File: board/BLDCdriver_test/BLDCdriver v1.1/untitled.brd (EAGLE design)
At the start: 46 x 65 mm, 26 parts, among them M1 JST-XH-03-PIN-LONG-PAD, X1 JST-XH-02-PIN-LONG-PAD, X2 JST-XH-06-PIN-ROUND-PAD, X4 JST-XH-04-PIN-ROUND-PAD

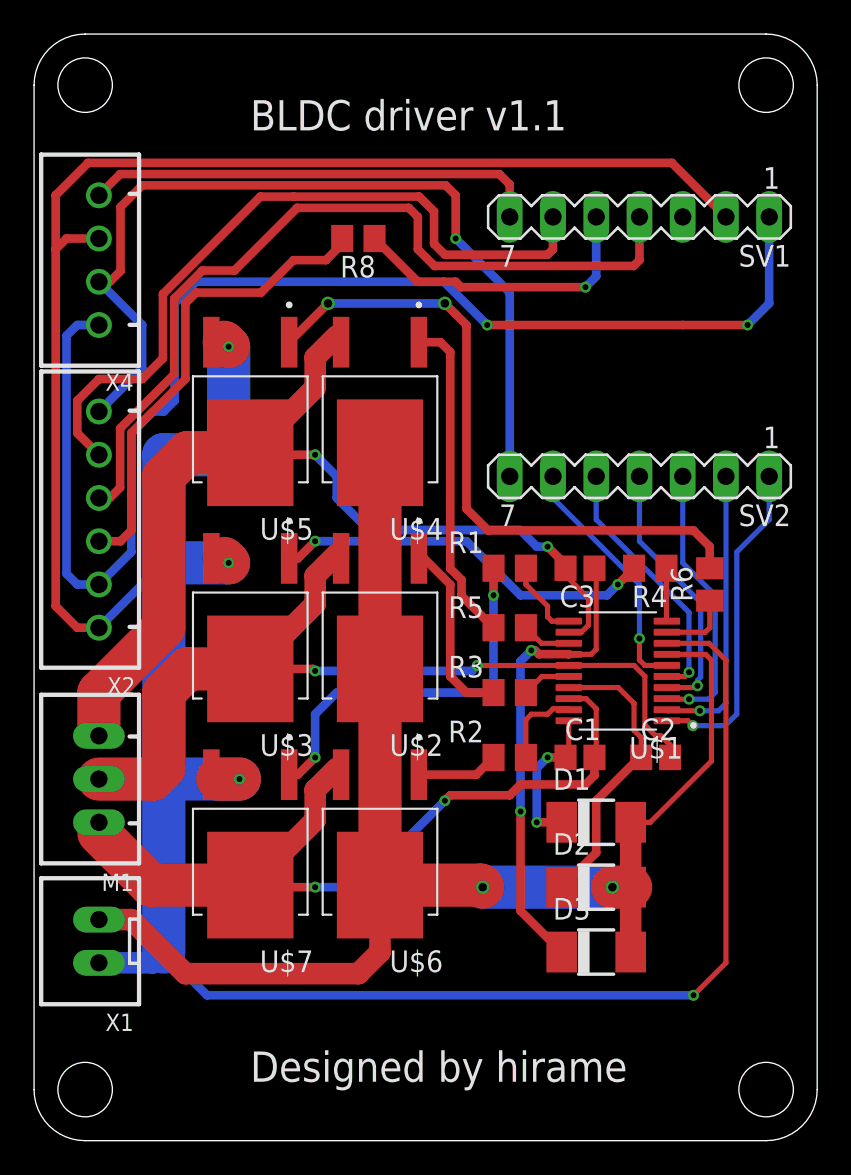
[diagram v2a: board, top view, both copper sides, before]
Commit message: Revert "Merge remote-tracking branch 'origin/Develop' into feature_#37"
This reverts commit cb103155361e8766478c6830db153463370c0739, reversing
changes made to 84e093fe944e1f8653a6822ff34e6f8740617cb5.
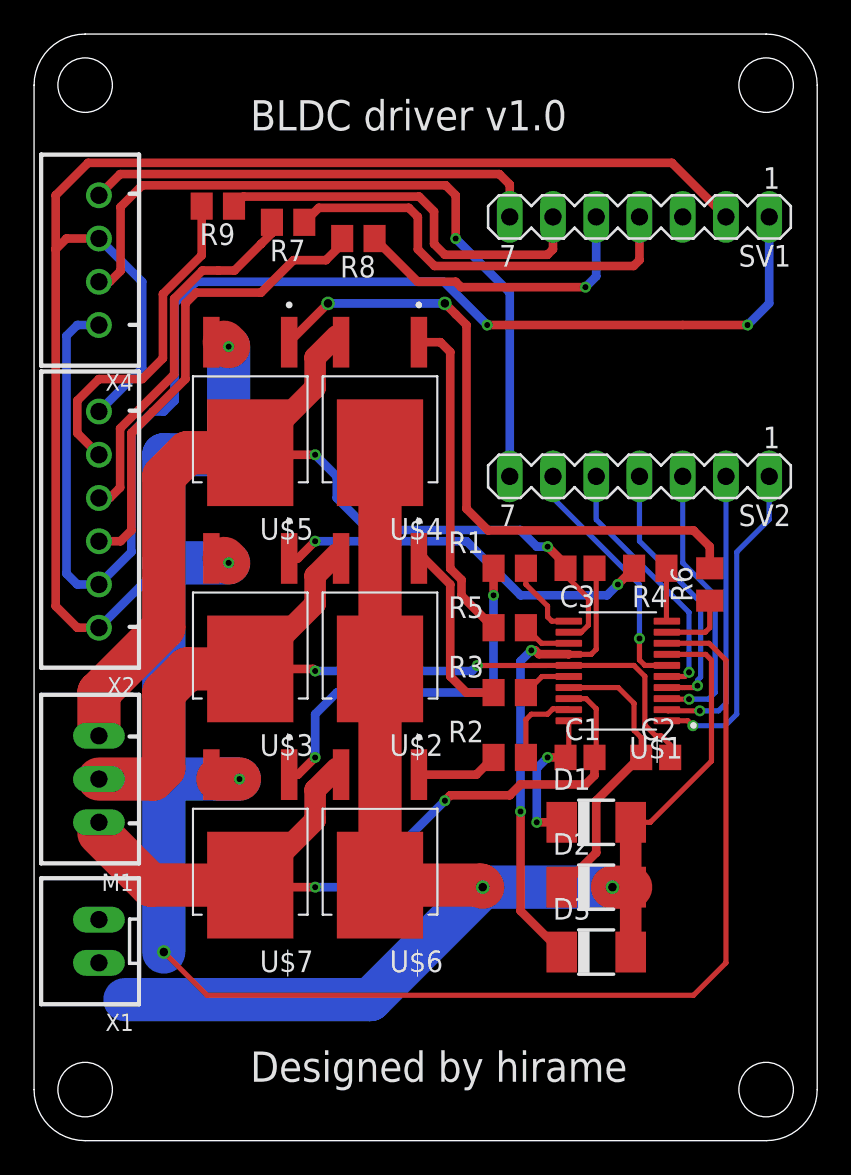
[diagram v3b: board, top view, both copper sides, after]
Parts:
- added R7, R9: 300Ω, adafruit:M2012
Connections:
- new net N$11: R7.1, SV1.4
- new net N$20: R9.1, SV1.6
- net GND: now also X2.6
- net MOSI: now also R7.2; no longer SV1.4
- net SCK: now also R9.2; no longer SV1.6
- net TX: no longer X2.6
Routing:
- net MOSI: track 48.7 -> 21.9 mm
- net N$11: track 0.00 -> 25.3 mm
- net SCK: track 43.4 -> 19.6 mm
- net N$20: track 0.00 -> 23.5 mm
- net TX: track 53.3 -> 43.6 mm
- net GND: track 188.7 -> 196.9 mm
- net VCC: track 85.0 -> 86.5 mm
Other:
- board text added: "BLDC driver v1.0"
- board text removed: "BLDC driver v1.1"
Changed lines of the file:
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@@
 <?xml version="1.0" encoding="utf-8"?>
 <!DOCTYPE eagle SYSTEM "eagle.dtd">
-<eagle version="9.6.2">
+<eagle version="9.6.1">
 <drawing>
 <settings>
@@
 <wire x1="43" y1="-6" x2="46" y2="-3" width="0.001" layer="20" curve="90"/>
 <text x="12.7" y="-2.54" size="1.778" layer="25" font="vector">Designed by hirame</text>
-<text x="12.7" y="53.34" size="1.778" layer="25" font="vector">BLDC driver v1.1</text>
+<text x="12.7" y="53.34" size="1.778" layer="25" font="vector">BLDC driver v1.0</text>
 </plain>
 <attributes>
@@
 <attribute name="VALUE" x="-0.0825" y="39.7175" size="1.016" layer="27" ratio="10" rot="R90"/>
 </element>
+<element name="R7" library="adafruit" package="M2012" value="300Ω" x="14.9225" y="47.9425" smashed="yes" rot="R180">
+<attribute name="NAME" x="15.9385" y="46.9265" size="1.27" layer="25" rot="R180"/>
+<attribute name="VALUE" x="15.9385" y="50.2285" size="1.27" layer="27" rot="R180"/>
+</element>
 <element name="R8" library="adafruit" package="M2012" value="300Ω" x="19.05" y="46.99" smashed="yes" rot="R180">
 <attribute name="NAME" x="20.066" y="45.974" size="1.27" layer="25" rot="R180"/>
 <attribute name="VALUE" x="20.066" y="49.276" size="1.27" layer="27" rot="R180"/>
+</element>
+<element name="R9" library="adafruit" package="M2012" value="300Ω" x="10.795" y="48.895" smashed="yes" rot="R180">
+<attribute name="NAME" x="11.811" y="47.879" size="1.27" layer="25" rot="R180"/>
+<attribute name="VALUE" x="11.811" y="51.181" size="1.27" layer="27" rot="R180"/>
 </element>
 </elements>
@@
 <contactref element="U$5" pad="3"/>
 <contactref element="U$1" pad="8"/>
-<wire x1="7.62" y1="15.24" x2="7.62" y2="5.08" width="2.54" layer="16"/>
+<via x="7.62" y="5.08" extent="1-16" drill="0.5"/>
+<wire x1="7.62" y1="5.08" x2="7.62" y2="15.24" width="2.54" layer="16"/>
 <wire x1="7.62" y1="15.24" x2="7.62" y2="27.94" width="2.54" layer="16"/>
 <contactref element="SV1" pad="2"/>
@@
 <wire x1="39.65" y1="23.215" x2="40.64" y2="22.225" width="0.3048" layer="1"/>
 <wire x1="40.64" y1="22.225" x2="40.64" y2="4.445" width="0.3048" layer="1"/>
+<wire x1="38.735" y1="2.54" x2="10.16" y2="2.54" width="0.3048" layer="1"/>
+<wire x1="10.16" y1="2.54" x2="7.62" y2="5.08" width="0.3048" layer="1"/>
 <wire x1="11.17" y1="40.9" x2="10.414" y2="40.9" width="0.3048" layer="1"/>
 <via x="11.43" y="40.64" extent="1-16" drill="0.35"/>
@@
 <wire x1="7.62" y1="34.29" x2="7.62" y2="27.94" width="2.54" layer="16"/>
 <wire x1="10.414" y1="15.5" x2="10.535" y2="15.5" width="0.508" layer="1"/>
+<contactref element="X2" pad="6"/>
+<wire x1="3.81" y1="46.99" x2="6.35" y2="44.45" width="0.508" layer="16"/>
+<wire x1="6.35" y1="39.37" x2="3.81" y2="36.83" width="0.508" layer="16"/>
+<wire x1="6.35" y1="44.45" x2="6.35" y2="39.37" width="0.508" layer="16"/>
 <contactref element="X1" pad="1"/>
-<wire x1="3.81" y1="4.445" x2="6.985" y2="4.445" width="1.27" layer="16"/>
-<wire x1="6.985" y1="4.445" x2="7.62" y2="5.08" width="1.27" layer="16"/>
-<wire x1="7.62" y1="5.08" x2="10.16" y2="2.54" width="0.508" layer="16"/>
-<wire x1="10.16" y1="2.54" x2="38.735" y2="2.54" width="0.508" layer="16"/>
-<via x="38.735" y="2.54" extent="1-16" drill="0.35"/>
+<wire x1="3.81" y1="4.445" x2="7.62" y2="5.08" width="0" layer="19" extent="1-1"/>
 </signal>
 <signal name="N$12">
@@
 <wire x1="39.7891" y1="22.225" x2="39.7891" y2="16.2941" width="0.3048" layer="1"/>
 <wire x1="39.7891" y1="16.2941" x2="36.195" y2="12.7" width="0.3048" layer="1"/>
+<wire x1="19.7485" y1="2.286" x2="26.3525" y2="8.89" width="2.54" layer="16"/>
+<wire x1="5.334" y1="2.286" x2="19.7485" y2="2.286" width="2.54" layer="16"/>
 <contactref element="X1" pad="2"/>
-<wire x1="3.81" y1="6.985" x2="5.715" y2="6.985" width="1.27" layer="1"/>
-<wire x1="8.89" y1="3.81" x2="19.05" y2="3.81" width="1.27" layer="1"/>
-<wire x1="19.05" y1="3.81" x2="20.32" y2="5.08" width="1.27" layer="1"/>
-<wire x1="20.32" y1="5.08" x2="20.32" y2="9.01" width="1.27" layer="1"/>
-<wire x1="5.715" y1="6.985" x2="8.89" y2="3.81" width="1.27" layer="1"/>
+<wire x1="5.334" y1="2.286" x2="3.81" y2="6.985" width="0" layer="19" extent="16-16"/>
 </signal>
 <signal name="N$15">
@@
 <wire x1="5.0546" y1="35.83355" x2="8.2296" y2="39.00855" width="0.508" layer="1"/>
 <wire x1="8.2296" y1="39.00855" x2="8.2296" y2="43.45355" width="0.508" layer="1"/>
-<wire x1="9.88645" y1="45.1104" x2="11.7729" y2="45.1104" width="0.508" layer="1"/>
-<contactref element="SV1" pad="4"/>
-<wire x1="22.0091" y1="48.7934" x2="22.5425" y2="48.26" width="0.508" layer="1"/>
-<wire x1="35.2171" y1="45.3771" x2="35.56" y2="45.72" width="0.508" layer="1"/>
-<wire x1="35.56" y1="45.72" x2="35.56" y2="48.26" width="0.508" layer="1"/>
-<wire x1="22.5425" y1="48.26" x2="22.5425" y2="46.355" width="0.508" layer="1"/>
-<wire x1="22.5425" y1="46.355" x2="23.5204" y2="45.3771" width="0.508" layer="1"/>
-<wire x1="23.5204" y1="45.3771" x2="35.2171" y2="45.3771" width="0.508" layer="1"/>
-<wire x1="15.4559" y1="48.7934" x2="22.0091" y2="48.7934" width="0.508" layer="1"/>
-<wire x1="11.7729" y1="45.1104" x2="15.4559" y2="48.7934" width="0.508" layer="1"/>
+<contactref element="R7" pad="2"/>
+<wire x1="13.9725" y1="47.31" x2="13.9725" y2="47.9425" width="0.508" layer="1"/>
+<wire x1="9.88645" y1="45.1104" x2="10.8204" y2="45.1104" width="0.508" layer="1"/>
+<wire x1="13.335" y1="46.6725" x2="13.9725" y2="47.31" width="0.508" layer="1"/>
+<wire x1="10.8204" y1="45.1104" x2="11.7729" y2="45.1104" width="0.508" layer="1"/>
+<wire x1="11.7729" y1="45.1104" x2="13.335" y2="46.6725" width="0.508" layer="1"/>
 </signal>
 <signal name="SCK">
@@
 <wire x1="2.54" y1="37.465" x2="3.81" y2="38.735" width="0.508" layer="1"/>
 <wire x1="7.5692" y1="39.9542" x2="7.5692" y2="43.7271" width="0.508" layer="1"/>
-<contactref element="SV1" pad="6"/>
-<wire x1="22.6187" y1="49.4538" x2="23.495" y2="48.5775" width="0.508" layer="1"/>
-<wire x1="23.495" y1="46.6725" x2="24.13" y2="46.0375" width="0.508" layer="1"/>
-<wire x1="30.1625" y1="46.0375" x2="30.48" y2="46.355" width="0.508" layer="1"/>
-<wire x1="30.48" y1="46.355" x2="30.48" y2="48.26" width="0.508" layer="1"/>
-<wire x1="15.24" y1="49.4538" x2="22.6187" y2="49.4538" width="0.508" layer="1"/>
-<wire x1="23.495" y1="48.5775" x2="23.495" y2="46.6725" width="0.508" layer="1"/>
-<wire x1="24.13" y1="46.0375" x2="30.1625" y2="46.0375" width="0.508" layer="1"/>
-<wire x1="13.2959" y1="49.4538" x2="15.24" y2="49.4538" width="0.508" layer="1"/>
-<wire x1="7.5692" y1="43.7271" x2="13.2959" y2="49.4538" width="0.508" layer="1"/>
+<contactref element="R9" pad="2"/>
+<wire x1="9.845" y1="46.0029" x2="9.845" y2="48.895" width="0.508" layer="1"/>
+<wire x1="7.5692" y1="43.7271" x2="9.845" y2="46.0029" width="0.508" layer="1"/>
 </signal>
 <signal name="RX">
@@
 <wire x1="5.08" y1="45.085" x2="5.08" y2="48.8442" width="0.508" layer="1"/>
 <wire x1="6.35" y1="50.1142" x2="24.1808" y2="50.1142" width="0.508" layer="1"/>
-<contactref element="X2" pad="6"/>
-<wire x1="6.35" y1="39.37" x2="6.35" y2="41.91" width="0.508" layer="16"/>
-<wire x1="6.35" y1="41.91" x2="3.81" y2="44.45" width="0.508" layer="16"/>
-<wire x1="3.81" y1="36.83" x2="6.35" y2="39.37" width="0.508" layer="16"/>
 </signal>
 <signal name="LC">
@@
 <wire x1="41.275" y1="19.05" x2="41.275" y2="28.575" width="0.3048" layer="16"/>
 </signal>
+<signal name="N$11">
+<contactref element="SV1" pad="4"/>
+<contactref element="R7" pad="1"/>
+<wire x1="15.8725" y1="47.9425" x2="16.7234" y2="48.7934" width="0.508" layer="1"/>
+<wire x1="22.0091" y1="48.7934" x2="22.5425" y2="48.26" width="0.508" layer="1"/>
+<wire x1="35.2171" y1="45.3771" x2="35.56" y2="45.72" width="0.508" layer="1"/>
+<wire x1="35.56" y1="45.72" x2="35.56" y2="48.26" width="0.508" layer="1"/>
+<wire x1="16.7234" y1="48.7934" x2="22.0091" y2="48.7934" width="0.508" layer="1"/>
+<wire x1="22.5425" y1="48.26" x2="22.5425" y2="46.355" width="0.508" layer="1"/>
+<wire x1="22.5425" y1="46.355" x2="23.5204" y2="45.3771" width="0.508" layer="1"/>
+<wire x1="23.5204" y1="45.3771" x2="35.2171" y2="45.3771" width="0.508" layer="1"/>
+</signal>
+<signal name="N$20">
+<contactref element="SV1" pad="6"/>
+<contactref element="R9" pad="1"/>
+<wire x1="11.745" y1="48.895" x2="12.3038" y2="49.4538" width="0.508" layer="1"/>
+<wire x1="22.6187" y1="49.4538" x2="23.495" y2="48.5775" width="0.508" layer="1"/>
+<wire x1="23.495" y1="46.6725" x2="24.13" y2="46.0375" width="0.508" layer="1"/>
+<wire x1="30.1625" y1="46.0375" x2="30.48" y2="46.355" width="0.508" layer="1"/>
+<wire x1="30.48" y1="46.355" x2="30.48" y2="48.26" width="0.508" layer="1"/>
+<wire x1="12.3038" y1="49.4538" x2="22.6187" y2="49.4538" width="0.508" layer="1"/>
+<wire x1="23.495" y1="48.5775" x2="23.495" y2="46.6725" width="0.508" layer="1"/>
+<wire x1="24.13" y1="46.0375" x2="30.1625" y2="46.0375" width="0.508" layer="1"/>
+</signal>
 <signal name="N$21">
